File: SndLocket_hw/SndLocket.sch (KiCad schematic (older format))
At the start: 226 parts, among them M1 MOTOR_NO_CONTACTS, Q1 IRLML6401, Q2 IRLML6401, Q3 IRLML6401, Q4 IRLML6401, Q5 TEMT7000, Q6 TSOP4856, Q7 LED_RGB 5050, Q8 IRLML6401, Q9 MMBT2222, SW1 SWITCH, SW2 DIPx8, SW3 BUTTON, SW4 BUTTON, SW5 BUTTON

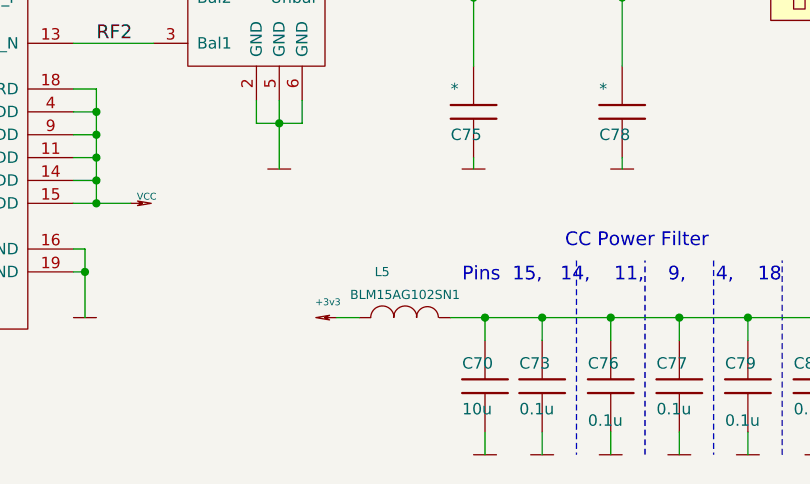
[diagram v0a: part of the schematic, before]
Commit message: Proceeding w os adaptation
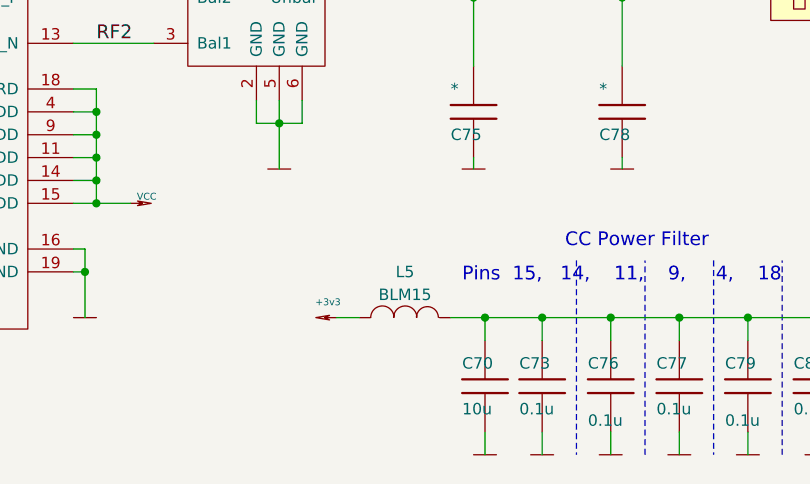
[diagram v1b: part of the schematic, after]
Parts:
- L5: value BLM15AG102SN1 -> BLM15; PN (none) -> SBY100505T-102Y-N; Price (none) -> 1; SolderPoints (none) -> 2
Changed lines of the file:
@@
 Wire Wire Line
 	17950 15850 17950 15950
-$Comp
-L Tittar_kl:L L5
-U 1 1 5DFFF98E
-P 15850 15350
-F 0 "L5" V 16050 15250 40  0000 C CNN
-F 1 "BLM15AG102SN1" V 15950 15350 40  0000 C CNN
-F 2 "Inductors:IND_0402" V 15910 15360 40  0001 C CNN
-F 3 "" H 15850 15350 60  0000 C CNN
-	1    15850 15350
-	0    1    -1   0
-$EndComp
 Wire Wire Line
 	18100 15350 18200 15350
@@
 Text Label 1800 3950 0    60   ~ 0
 DIP8
-Wire Bus Line
-	7300 3250 7300 5000
-Wire Bus Line
-	12400 13450 12400 14550
 Text Label 1800 3650 0    60   ~ 0
 DIP5
+$Comp
+L Tittar_kl:L L5
+U 1 1 5C828D04
+P 15850 15350
+F 0 "L5" V 16050 15350 50  0000 C CNN
+F 1 "BLM15" V 15950 15350 50  0000 C CNN
+F 2 "Inductors:IND_0402" V 15910 15360 40  0001 C CNN
+F 3 "" V 15750 15210 60  0001 C CNN
+F 4 "1" V 15850 15310 60  0001 C CNN "Price"
+F 5 "2" V 15950 15410 60  0001 C CNN "SolderPoints"
+F 6 "SBY100505T-102Y-N" V 15850 15350 50  0001 C CNN "PN"
+	1    15850 15350
+	0    1    -1   0
+$EndComp
+Wire Bus Line
+	12400 13450 12400 14550
+Wire Bus Line
+	7300 3250 7300 5000
 $EndSCHEMATC
